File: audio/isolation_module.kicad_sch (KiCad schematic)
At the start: 16 parts, among them J8 Conn_01x10, J9 Conn_01x10, U2 ISO1540, U9 SI8663BB-B-IS1

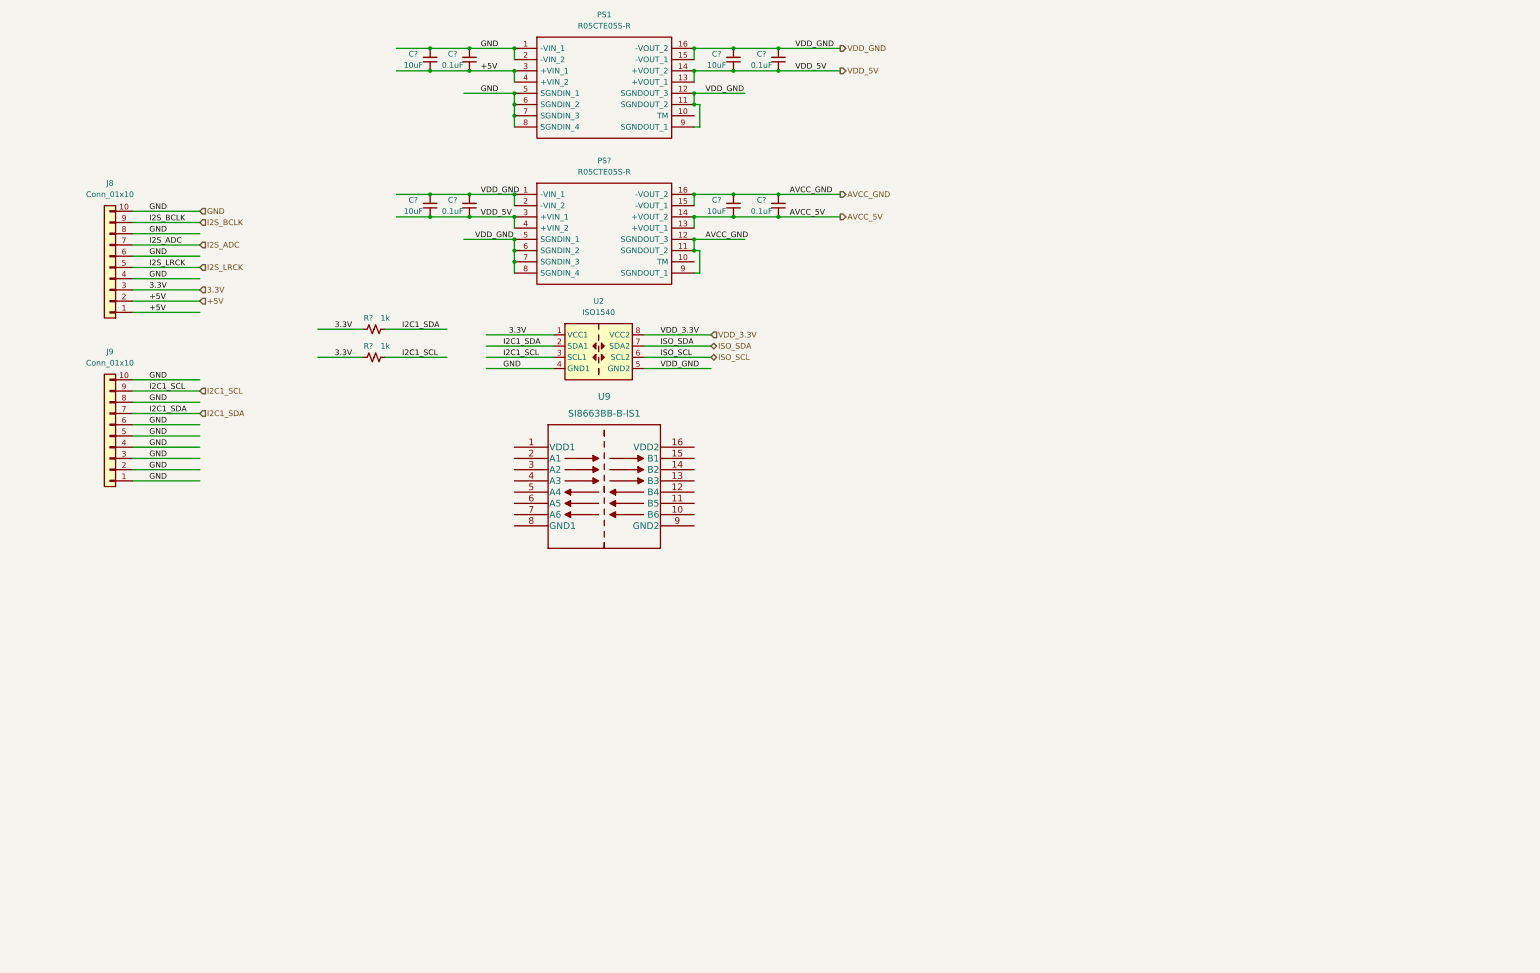
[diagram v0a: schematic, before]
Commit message: .
.
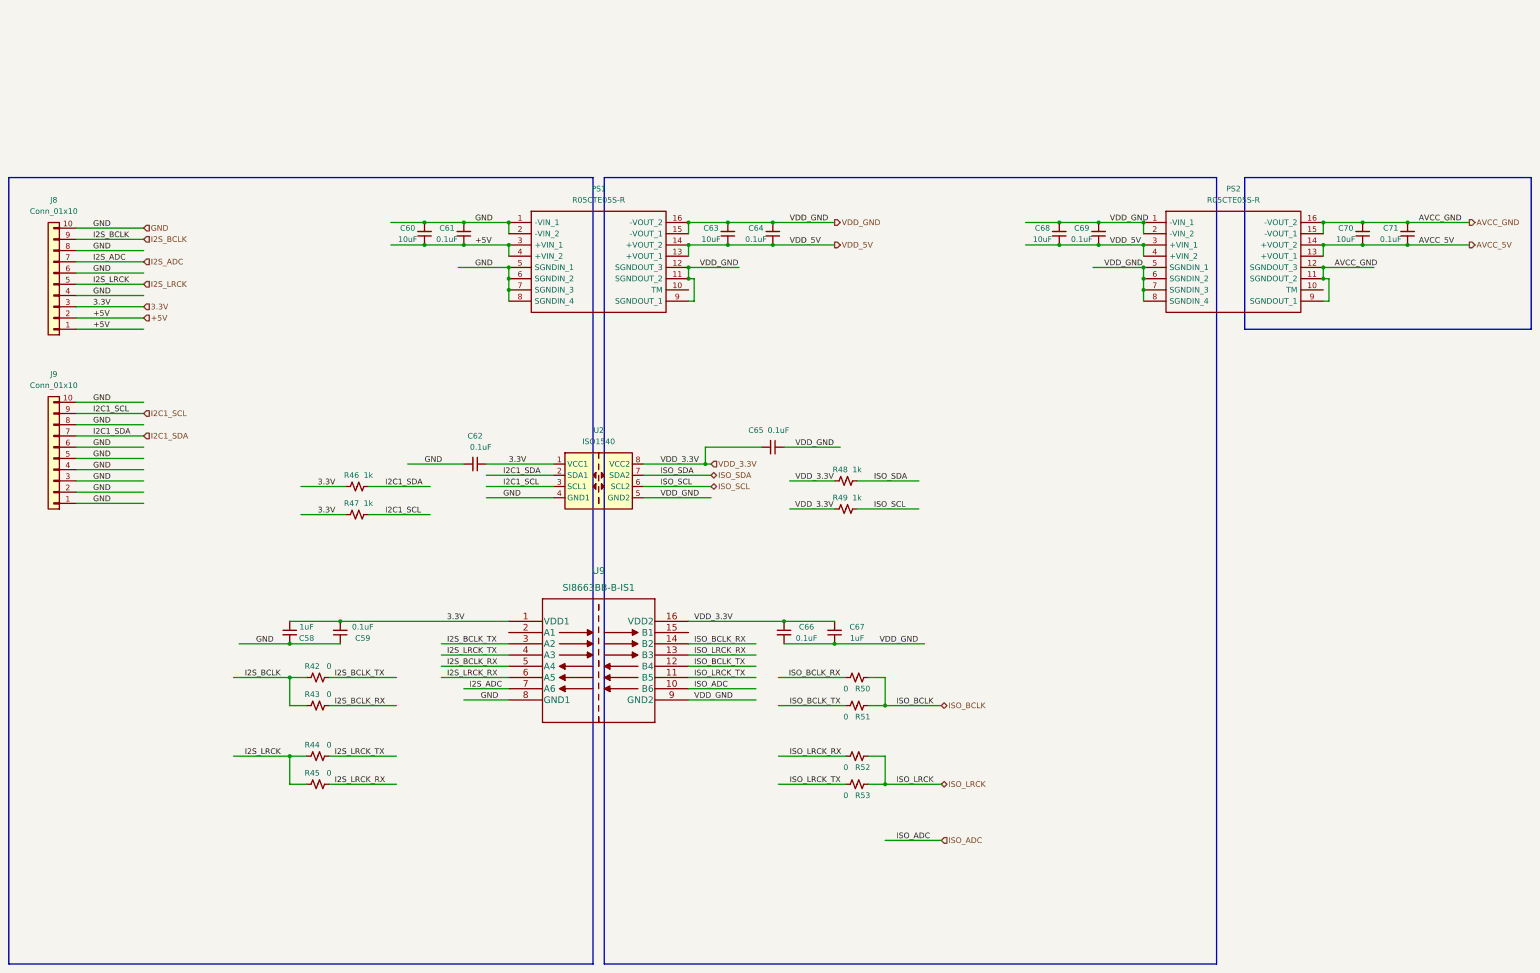
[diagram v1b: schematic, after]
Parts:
- added C58, C67: 1uF, Capacitor_SMD:C_0402_1005Metric, symbol Device:C_Small
- added C59, C62, C65, C66: 0.1uF, Capacitor_SMD:C_0402_1005Metric, symbol Device:C_Small
- added R42, R43, R44, R45, R50, R51, R52, R53: 0, Resistor_SMD:R_0603_1608Metric, symbol Device:R_Small_US
- added R48, R49: 1k, Resistor_SMD:R_0603_1608Metric, symbol Device:R_Small_US
- gave numbers to parts that had none: 11
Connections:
- net 3.3V: now also U9.1 (VDD1), C58.1, C59.2, C62.1
- net GND: now also U9.8 (GND1), C58.2, C59.1, C62.2
- net I2S_ADC: now also U9.7 (A6)
- net I2S_BCLK: now also R42.1, R43.1
- net I2S_LRCK: now also R44.1, R45.1
- net ISO_SCL: now also R49.2
- net ISO_SDA: now also R48.2
- net VDD_3.3V: now also U9.16 (VDD2), C65.2, C66.1, C67.2, R48.1, R49.1
- net VDD_GND: now also U9.9 (GND2), C65.1, C66.2, C67.1
- net ISO_ADC: now reaches U9.10 (B6)
- net ISO_LRCK_TX: now reaches U9.11 (B5)
- net ISO_LRCK_TX: now also R53.2
- net ISO_BCLK_TX: now reaches U9.12 (B4)
- net ISO_BCLK_TX: now also R51.2
- net ISO_LRCK_RX: now reaches U9.13 (B3)
- net ISO_LRCK_RX: now also R52.2
- net ISO_BCLK_RX: now reaches U9.14 (B2)
- net ISO_BCLK_RX: now also R50.2
- net I2S_BCLK_TX: now reaches U9.3 (A2)
- net I2S_BCLK_TX: now also R42.2
- net I2S_LRCK_TX: now reaches U9.4 (A3)
- net I2S_LRCK_TX: now also R44.2
- net I2S_BCLK_RX: now reaches U9.5 (A4)
- net I2S_BCLK_RX: now also R43.2
- net I2S_LRCK_RX: now reaches U9.6 (A5)
- net I2S_LRCK_RX: now also R45.2
- new net ISO_BCLK: R50.1, R51.1
- new net ISO_LRCK: R52.1, R53.1
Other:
- moved on the sheet: C60, C61, C63, C64, C68, C69, C70, C71, J8, J9, PS1, PS2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
